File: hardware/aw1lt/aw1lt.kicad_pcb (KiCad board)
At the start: 2 copper layers, 30 x 22 mm, 29 parts, among them J1 ISP_FTDI, Q1 Q_NPN_CBE, SW1 SW_Push, SW2 SW_Push, SW3 SW_Push, U1 DS3231MZ, U2 ATMEGA328P-AU

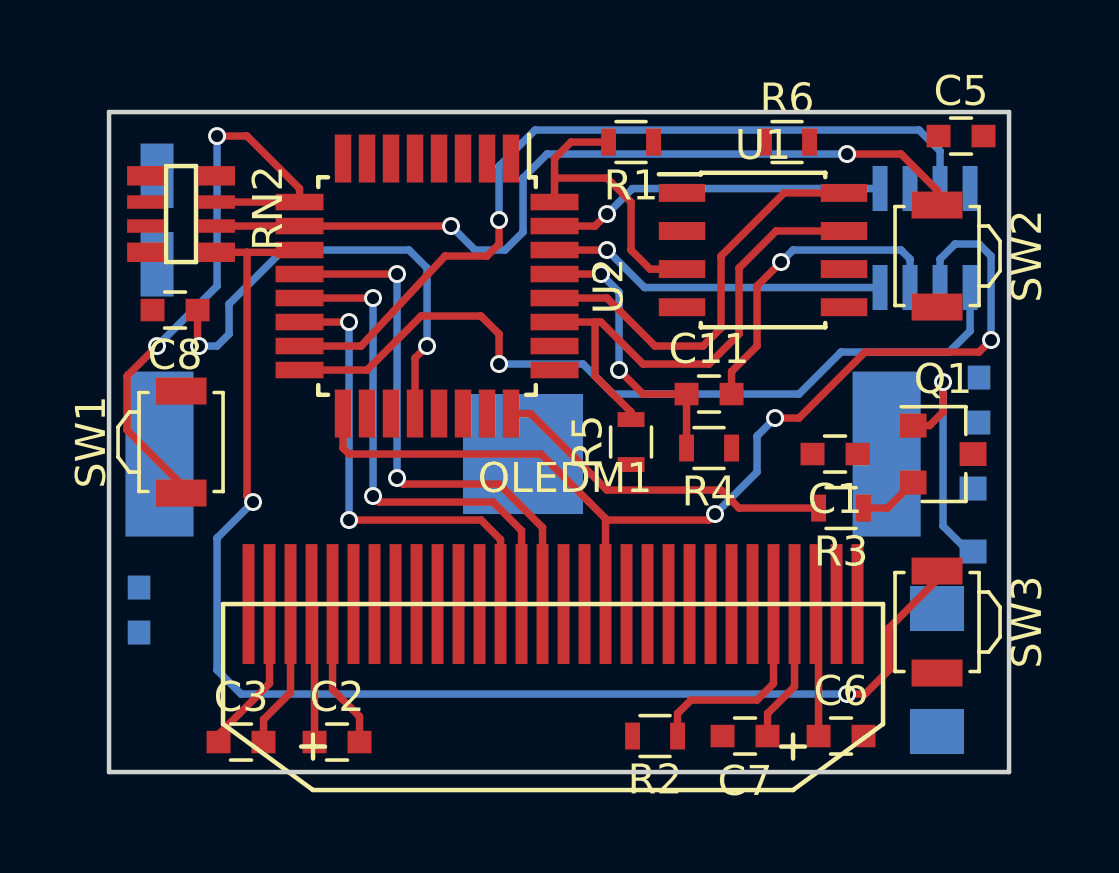
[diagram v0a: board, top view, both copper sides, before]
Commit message: some changes
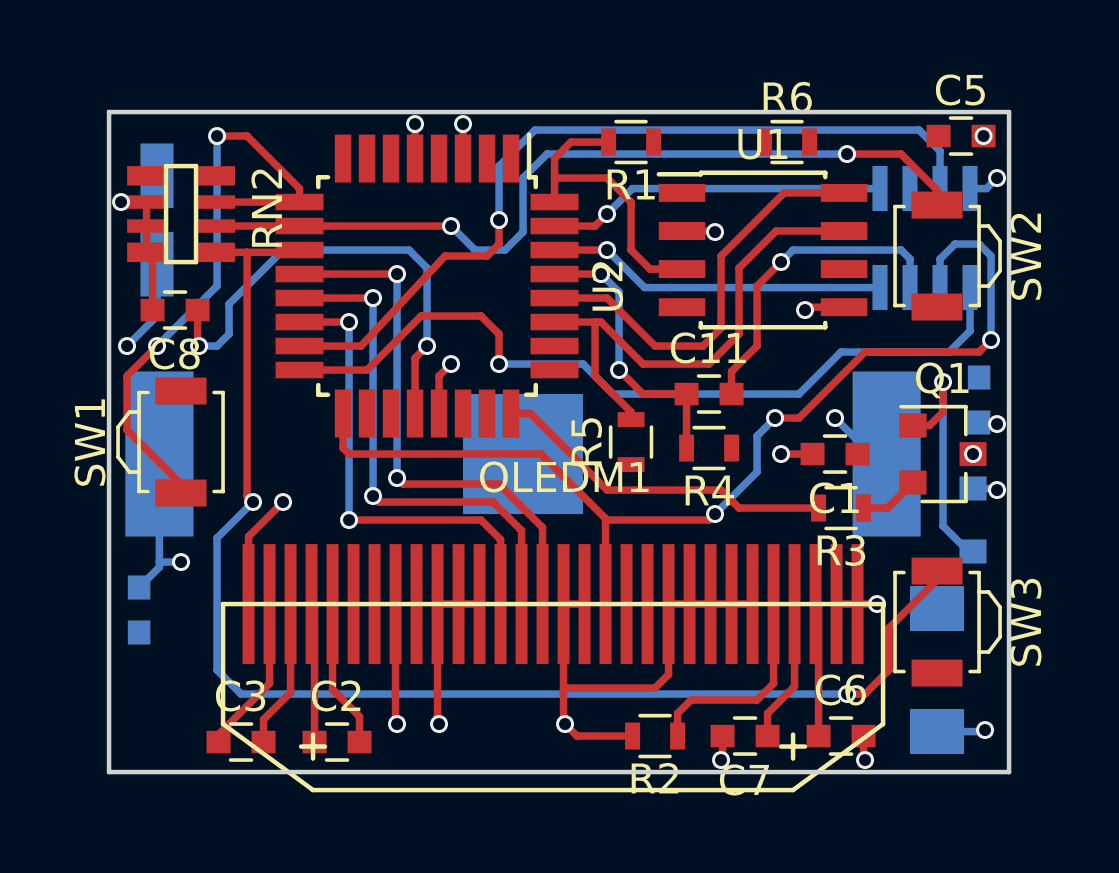
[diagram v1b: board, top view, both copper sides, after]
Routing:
- net GND: track 0.00 -> 44.5 mm, vias 0 -> 16
- net +3V3: track 0.00 -> 14.9 mm, vias 0 -> 7
- added copper zone on F.Cu, net +3V3
- added copper zone on B.Cu, net GND
